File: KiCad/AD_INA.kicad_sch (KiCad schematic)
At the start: 7 parts, among them U2 AD623/INA126

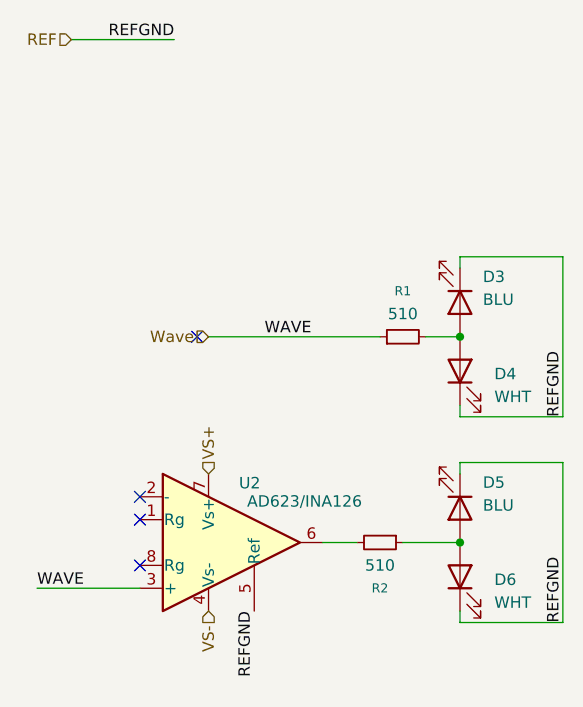
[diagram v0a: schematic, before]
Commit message: added footprints to schematic
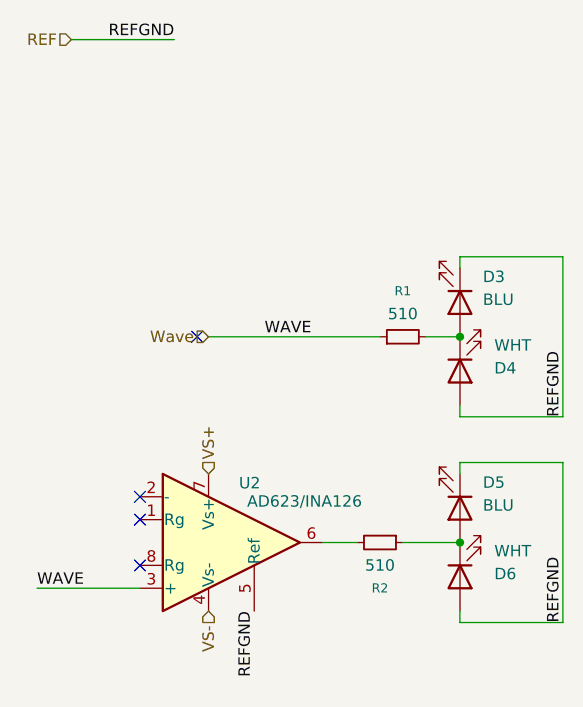
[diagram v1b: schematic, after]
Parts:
- D3, D4, D5, D6: footprint (none) -> Diode_SMD:D_0201_0603Metric
- R1, R2: footprint (none) -> Resistor_SMD:R_0201_0603Metric
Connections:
- net REF: now also D4.2 (A), D6.2 (A); no longer D4.1 (K), D6.1 (K)
- net at D3.2 (A), R1.2: now also D4.1 (K); no longer D4.2 (A)
- net at D5.2 (A), R2.1: now also D6.1 (K); no longer D6.2 (A)
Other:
- moved on the sheet: D4, D6
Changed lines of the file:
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@@
 			)
 		)
-		(property "Footprint" ""
+		(property "Footprint" "Diode_SMD:D_0201_0603Metric"
 			(at 64.77 58.42 0)
 			(effects
@@
 			)
 		)
-		(property "Footprint" ""
+		(property "Footprint" "Resistor_SMD:R_0201_0603Metric"
 			(at 58.42 62.23 0)
 			(effects
@@
 		(lib_id "Device:LED")
 		(at 64.77 88.9 90)
-		(unit 1)
-		(exclude_from_sim no)
-		(in_bom yes)
-		(on_board yes)
-		(dnp no)
-		(fields_autoplaced yes)
+		(mirror x)
+		(unit 1)
+		(exclude_from_sim no)
+		(in_bom yes)
+		(on_board yes)
+		(dnp no)
 		(property "Reference" "D6"
-			(at 68.58 89.2174 90)
+			(at 68.58 88.5826 90)
 			(effects
 				(font
@@
 		)
 		(property "Value" "WHT"
-			(at 68.58 91.7574 90)
+			(at 68.58 86.0426 90)
 			(effects
 				(font
@@
 			)
 		)
-		(property "Footprint" ""
+		(property "Footprint" "Diode_SMD:D_0201_0603Metric"
 			(at 64.77 88.9 0)
 			(effects
@@
 			)
 		)
-		(property "Footprint" ""
+		(property "Footprint" "Diode_SMD:D_0201_0603Metric"
 			(at 64.77 81.28 0)
 			(effects
@@
 		(lib_id "Device:LED")
 		(at 64.77 66.04 90)
-		(unit 1)
-		(exclude_from_sim no)
-		(in_bom yes)
-		(on_board yes)
-		(dnp no)
-		(fields_autoplaced yes)
+		(mirror x)
+		(unit 1)
+		(exclude_from_sim no)
+		(in_bom yes)
+		(on_board yes)
+		(dnp no)
 		(property "Reference" "D4"
-			(at 68.58 66.3574 90)
+			(at 68.58 65.7226 90)
 			(effects
 				(font
@@
 		)
 		(property "Value" "WHT"
-			(at 68.58 68.8974 90)
+			(at 68.58 63.1826 90)
 			(effects
 				(font
@@
 			)
 		)
-		(property "Footprint" ""
+		(property "Footprint" "Diode_SMD:D_0201_0603Metric"
 			(at 64.77 66.04 0)
 			(effects
@@
 			)
 		)
-		(property "Footprint" ""
+		(property "Footprint" "Resistor_SMD:R_0201_0603Metric"
 			(at 55.88 85.09 0)
 			(effects

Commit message: Add power led
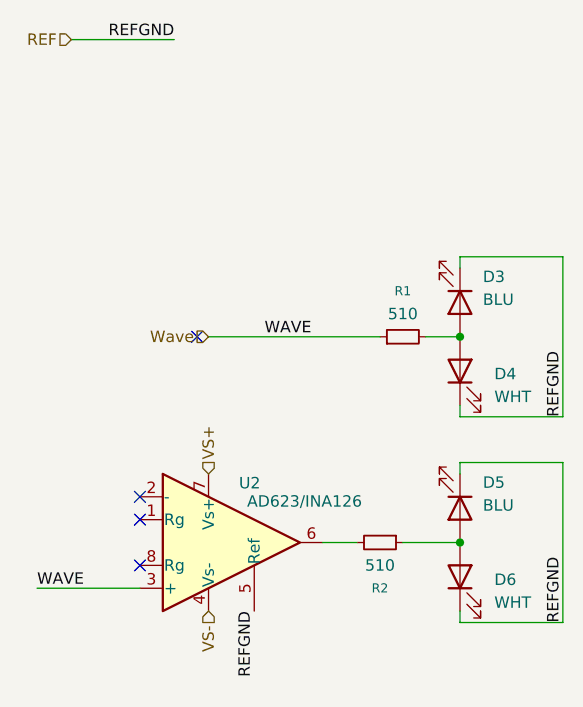
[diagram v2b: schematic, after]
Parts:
- D3, D4, D5, D6: footprint Diode_SMD:D_0201_0603Metric -> (none)
- R1, R2: footprint Resistor_SMD:R_0201_0603Metric -> (none)
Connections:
- net REF: now also D4.1 (K), D6.1 (K); no longer D4.2 (A), D6.2 (A)
- net at D3.2 (A), R1.2: now also D4.2 (A); no longer D4.1 (K)
- net at D5.2 (A), R2.1: now also D6.2 (A); no longer D6.1 (K)
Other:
- moved on the sheet: D4, D6
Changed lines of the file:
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@@
 			)
 		)
-		(property "Footprint" "Diode_SMD:D_0201_0603Metric"
+		(property "Footprint" ""
 			(at 64.77 58.42 0)
 			(effects
@@
 			)
 		)
-		(property "Footprint" "Resistor_SMD:R_0201_0603Metric"
+		(property "Footprint" ""
 			(at 58.42 62.23 0)
 			(effects
@@
 		(lib_id "Device:LED")
 		(at 64.77 88.9 90)
-		(mirror x)
-		(unit 1)
-		(exclude_from_sim no)
-		(in_bom yes)
-		(on_board yes)
-		(dnp no)
+		(unit 1)
+		(exclude_from_sim no)
+		(in_bom yes)
+		(on_board yes)
+		(dnp no)
+		(fields_autoplaced yes)
 		(property "Reference" "D6"
-			(at 68.58 88.5826 90)
+			(at 68.58 89.2174 90)
 			(effects
 				(font
@@
 		)
 		(property "Value" "WHT"
-			(at 68.58 86.0426 90)
+			(at 68.58 91.7574 90)
 			(effects
 				(font
@@
 			)
 		)
-		(property "Footprint" "Diode_SMD:D_0201_0603Metric"
+		(property "Footprint" ""
 			(at 64.77 88.9 0)
 			(effects
@@
 			)
 		)
-		(property "Footprint" "Diode_SMD:D_0201_0603Metric"
+		(property "Footprint" ""
 			(at 64.77 81.28 0)
 			(effects
@@
 		(lib_id "Device:LED")
 		(at 64.77 66.04 90)
-		(mirror x)
-		(unit 1)
-		(exclude_from_sim no)
-		(in_bom yes)
-		(on_board yes)
-		(dnp no)
+		(unit 1)
+		(exclude_from_sim no)
+		(in_bom yes)
+		(on_board yes)
+		(dnp no)
+		(fields_autoplaced yes)
 		(property "Reference" "D4"
-			(at 68.58 65.7226 90)
+			(at 68.58 66.3574 90)
 			(effects
 				(font
@@
 		)
 		(property "Value" "WHT"
-			(at 68.58 63.1826 90)
+			(at 68.58 68.8974 90)
 			(effects
 				(font
@@
 			)
 		)
-		(property "Footprint" "Diode_SMD:D_0201_0603Metric"
+		(property "Footprint" ""
 			(at 64.77 66.04 0)
 			(effects
@@
 			)
 		)
-		(property "Footprint" "Resistor_SMD:R_0201_0603Metric"
+		(property "Footprint" ""
 			(at 55.88 85.09 0)
 			(effects
